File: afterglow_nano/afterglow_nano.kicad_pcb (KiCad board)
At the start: 2 copper layers, 193.5 x 80 mm, 85 parts, among them J133 OUT J133_OUT_R, J134 OUT J134_OUT_R, J135 OUT J135_OUT_R, J136 OUT 136_OUT_C, J137 OUT J137_OUT_C, J138 OUT J138_OUT_C, J34 IN J133_IN_R, J38 IN J137_IN_C, Q1 2N3904, Q10 FQP27P06, Q11 FQP27P06, Q12 FQP27P06, Q13 FQP27P06, Q14 FQP27P06, Q15 FQP27P06, Q16 FQP27P06, Q17 FQP30N06L, Q18 FQP30N06L, Q19 FQP30N06L, Q2 2N3904, Q20 FQP30N06L, Q21 FQP30N06L, Q22 FQP30N06L, Q23 FQP30N06L, Q24 FQP30N06L, Q3 2N3904, Q4 2N3904, Q5 2N3904, Q6 2N3904, Q7 2N3904, Q8 2N3904, Q9 FQP27P06, U1 74LS165, U2 74LS165, U3 5V_Regulator, U4 arduino nano, U5 74HC595, U6 74HC595

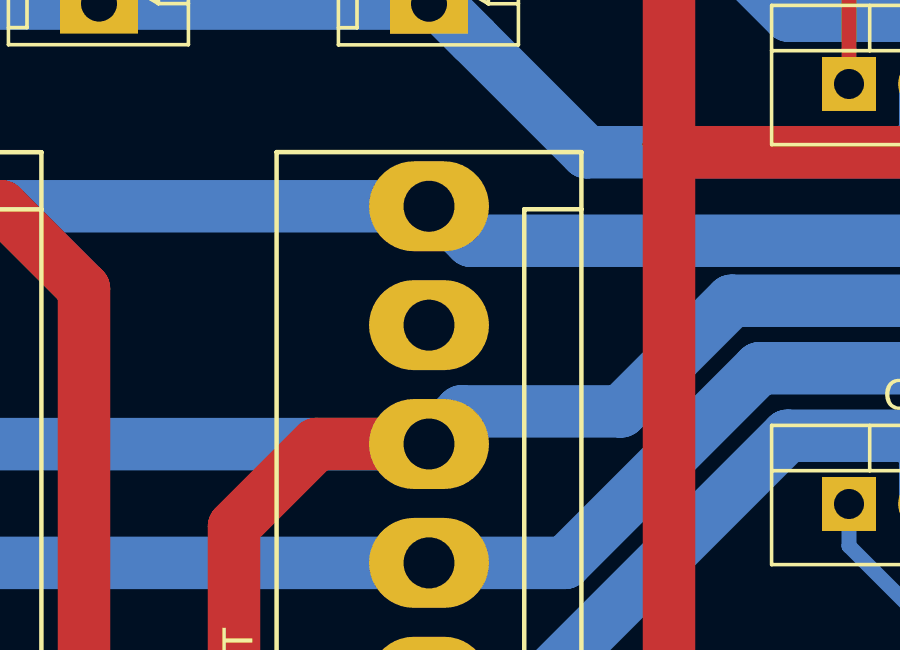
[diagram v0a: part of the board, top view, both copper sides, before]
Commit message: Minor trace fix
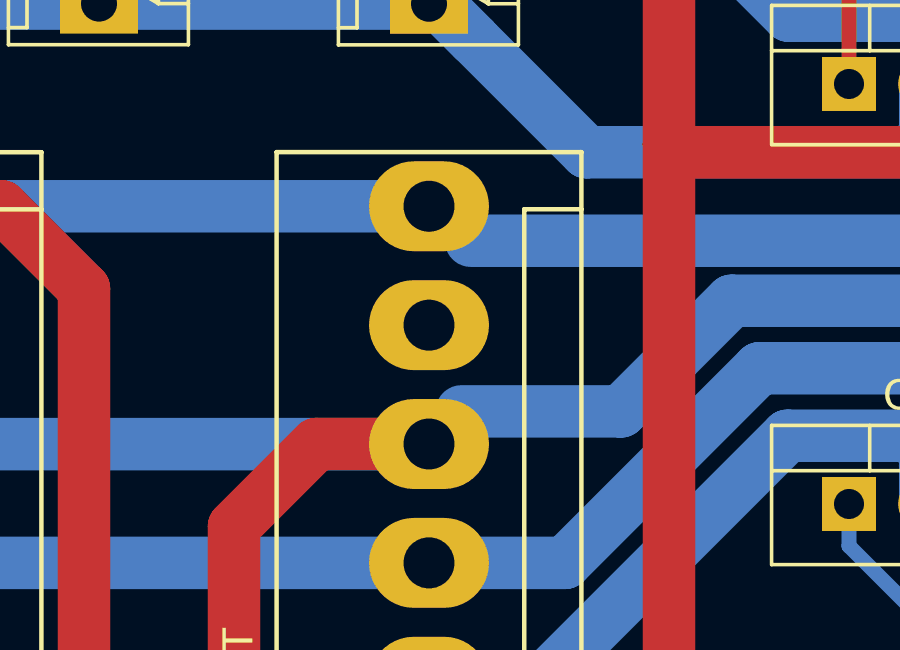
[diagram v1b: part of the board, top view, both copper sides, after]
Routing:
- net /J137_CO8: track 127.4 -> 125.8 mm
- net /J137_CO7: track 119.1 -> 117.5 mm
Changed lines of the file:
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@@
 (kicad_pcb (version 4) (host pcbnew 4.0.7)
   (general
-    (links 0)
-    (no_connects 26)
+    (links 240)
+    (no_connects 4)
     (area 17.571429 49.475 225.928572 130.625)
     (thickness 1.6)
     (drawings 31)
-    (tracks 1136)
+    (tracks 1135)
     (zones 0)
     (modules 85)
@@
   (segment (start 177.25 76.75) (end 178.5 75.5) (width 0.5) (layer F.Cu) (net 23))
   (segment (start 196.84 81.32) (end 196.8 81.28) (width 0.5) (layer F.Cu) (net 23))
+  (segment (start 60.603478 113.7744) (end 66.652879 107.724999) (width 1.75) (layer B.Cu) (net 24))
+  (segment (start 60 113.7744) (end 60.603478 113.7744) (width 1.75) (layer B.Cu) (net 24))
   (segment (start 42 113.7792) (end 59.9958 113.7792) (width 1.75) (layer B.Cu) (net 24))
   (segment (start 59.9958 113.7792) (end 60 113.775) (width 1.75) (layer B.Cu) (net 24))
   (segment (start 76.54 110) (end 88.38 98.16) (width 0.5) (layer F.Cu) (net 24))
   (segment (start 88.38 98.16) (end 88.38 98) (width 0.5) (layer F.Cu) (net 24))
-  (segment (start 60 113.7744) (end 60.603478 113.7744) (width 1.75) (layer B.Cu) (net 24))
   (segment (start 66.652879 107.724999) (end 75.621999 107.724999) (width 1.75) (layer B.Cu) (net 24))
-  (segment (start 60.603478 113.7744) (end 66.652879 107.724999) (width 1.75) (layer B.Cu) (net 24))
   (segment (start 76.54 108.727208) (end 76.54 110) (width 1.75) (layer B.Cu) (net 24))
   (segment (start 75.621999 107.724999) (end 76.54 108.643) (width 1.75) (layer B.Cu) (net 24))
   (segment (start 76.54 108.643) (end 76.54 108.727208) (width 1.75) (layer B.Cu) (net 24))
+  (segment (start 60.603478 109.812) (end 64.940489 105.474989) (width 1.75) (layer B.Cu) (net 25))
   (segment (start 60 109.8126) (end 42.0042 109.8126) (width 1.75) (layer B.Cu) (net 25))
   (segment (start 42.0042 109.8126) (end 42 109.8168) (width 1.75) (layer B.Cu) (net 25))
@@
   (segment (start 88 100.92) (end 90.92 98) (width 0.5) (layer F.Cu) (net 25))
   (segment (start 60 109.812) (end 60.603478 109.812) (width 1.75) (layer B.Cu) (net 25))
-  (segment (start 60.603478 109.812) (end 64.940489 105.474989) (width 1.75) (layer B.Cu) (net 25))
   (segment (start 64.940489 105.474989) (end 85.209991 105.474989) (width 1.75) (layer B.Cu) (net 25))
   (segment (start 85.209991 105.474989) (end 88 108.264998) (width 1.75) (layer B.Cu) (net 25))
@@
   (segment (start 85.209991 87.474989) (end 88 90.264998) (width 1.75) (layer B.Cu) (net 29))
   (segment (start 88 90.264998) (end 88 90.727208) (width 1.75) (layer B.Cu) (net 29))
+  (segment (start 60 90.0006) (end 60 90) (width 1.75) (layer F.Cu) (net 30))
   (segment (start 53.5 113.931994) (end 53.5 111.5) (width 1.75) (layer F.Cu) (net 30))
   (segment (start 53.5 111.5) (end 53.5 92.7506) (width 1.75) (layer F.Cu) (net 30))
@@
   (segment (start 99.46 92) (end 99.46 93.84) (width 0.5) (layer F.Cu) (net 30))
   (segment (start 99.46 93.84) (end 103.62 98) (width 0.5) (layer F.Cu) (net 30))
-  (segment (start 60 90) (end 61.08739 88.91261) (width 1.75) (layer B.Cu) (net 30))
   (segment (start 61.08739 88.91261) (end 66.398202 88.91261) (width 1.75) (layer B.Cu) (net 30))
   (segment (start 99.46 90.727208) (end 99.46 92) (width 1.75) (layer B.Cu) (net 30))
@@
   (segment (start 60 82.0752) (end 60.249924 82.0752) (width 1.75) (layer B.Cu) (net 32))
   (segment (start 61.399693 83.224969) (end 103.049971 83.224969) (width 1.75) (layer B.Cu) (net 32))
-  (segment (start 60.249924 82.0752) (end 61.399693 83.224969) (width 1.75) (layer B.Cu) (net 32))
   (segment (start 103.049971 83.224969) (end 110.54 90.714998) (width 1.75) (layer B.Cu) (net 32))
   (segment (start 110.54 90.714998) (end 110.54 90.727208) (width 1.75) (layer B.Cu) (net 32))
